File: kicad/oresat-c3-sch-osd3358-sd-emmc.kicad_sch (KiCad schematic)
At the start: 44 parts, among them J5 DM3BT-DSF-PEJS, U1 OSD3358-512M-BSM, U8 TCAN330, U9 EMMC+RESET+5.1-COMPATIBLE-BA

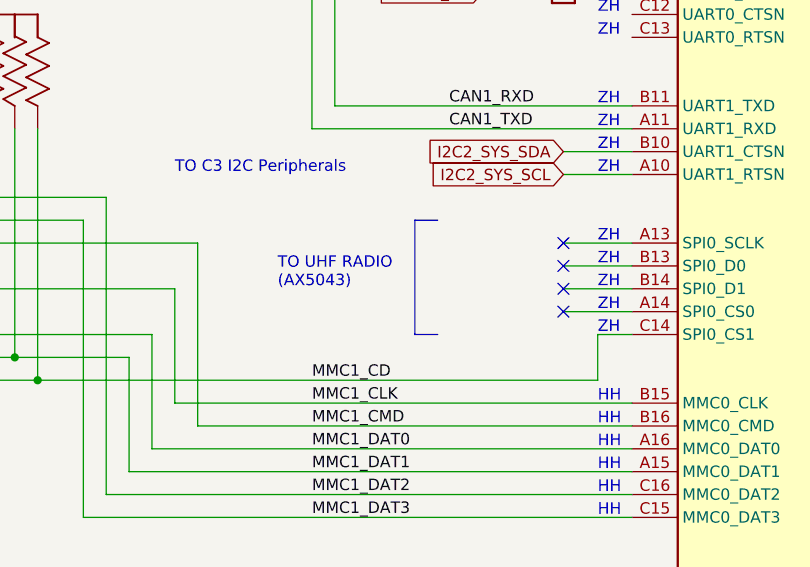
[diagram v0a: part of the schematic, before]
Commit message: Added I2C1 bus lines
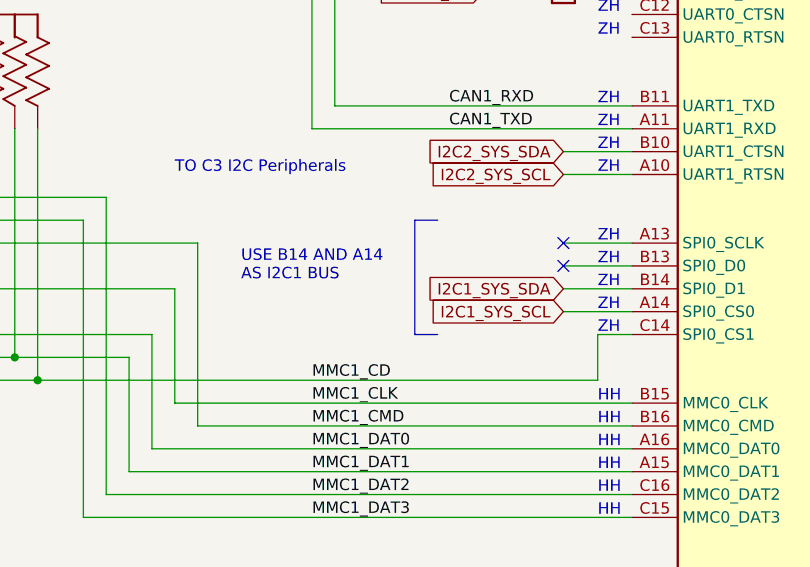
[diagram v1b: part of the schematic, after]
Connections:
- net I2C1_SYS_SCL: now reaches U1.A14 (SPI0_CS0)
- net I2C1_SYS_SDA: now reaches U1.B14 (SPI0_D1)
- no-connect marks 28 -> 26
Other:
- note added: "USE B14 AND A14 AS I2C1 BUS"
- note removed: "TO UHF RADIO (AX5043)"
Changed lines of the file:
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@@
 	)
 	(no_connect
-		(at 154.94 137.16)
-	)
-	(no_connect
 		(at 223.52 144.78)
 	)
@@
 	)
 	(no_connect
-		(at 154.94 139.7)
-	)
-	(no_connect
 		(at 154.94 177.8)
 	)
@@
 		)
 	)
-	(text "TO UHF RADIO\n(AX5043)"
+	(text "USE B14 AND A14 \nAS I2C1 BUS\n"
 		(exclude_from_sim no)
-		(at 123.19 137.16 0)
+		(at 119.126 136.398 0)
 		(effects
 			(font
@@
 		)
 	)
+	(global_label "I2C1_SYS_SDA"
+		(shape input)
+		(at 154.94 137.16 180)
+		(fields_autoplaced yes)
+		(effects
+			(font
+				(size 1.27 1.27)
+			)
+			(justify right)
+		)
+		(property "Intersheetrefs" "${INTERSHEET_REFS}"
+			(at 138.6501 137.16 0)
+			(effects
+				(font
+					(size 1.27 1.27)
+				)
+				(justify right)
+			)
+		)
+	)
 	(global_label "OPD_nENABLE"
 		(shape output)
@@
 			(effects
 				(font
+					(size 1.27 1.27)
+				)
+				(justify right)
+			)
+		)
+	)
+	(global_label "I2C1_SYS_SCL"
+		(shape input)
+		(at 154.94 139.7 180)
+		(fields_autoplaced yes)
+		(effects
+			(font
+				(size 1.27 1.27)
+			)
+			(justify right)
+		)
+		(property "Intersheetrefs" "${INTERSHEET_REFS}"
+			(at 138.7106 139.7 0)
+			(effects
+				(font
